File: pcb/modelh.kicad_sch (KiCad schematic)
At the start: 46 parts, among them J1 Battery Conn, J2 Conn_01x20, J3 Conn_01x05, J4 Conn_01x12, J5 Conn_01x04, J6 Conn_01x04, SW1 SW_reset, U1 nice_nano, U2 74HC595, U3 74HC595, U4 74HC595

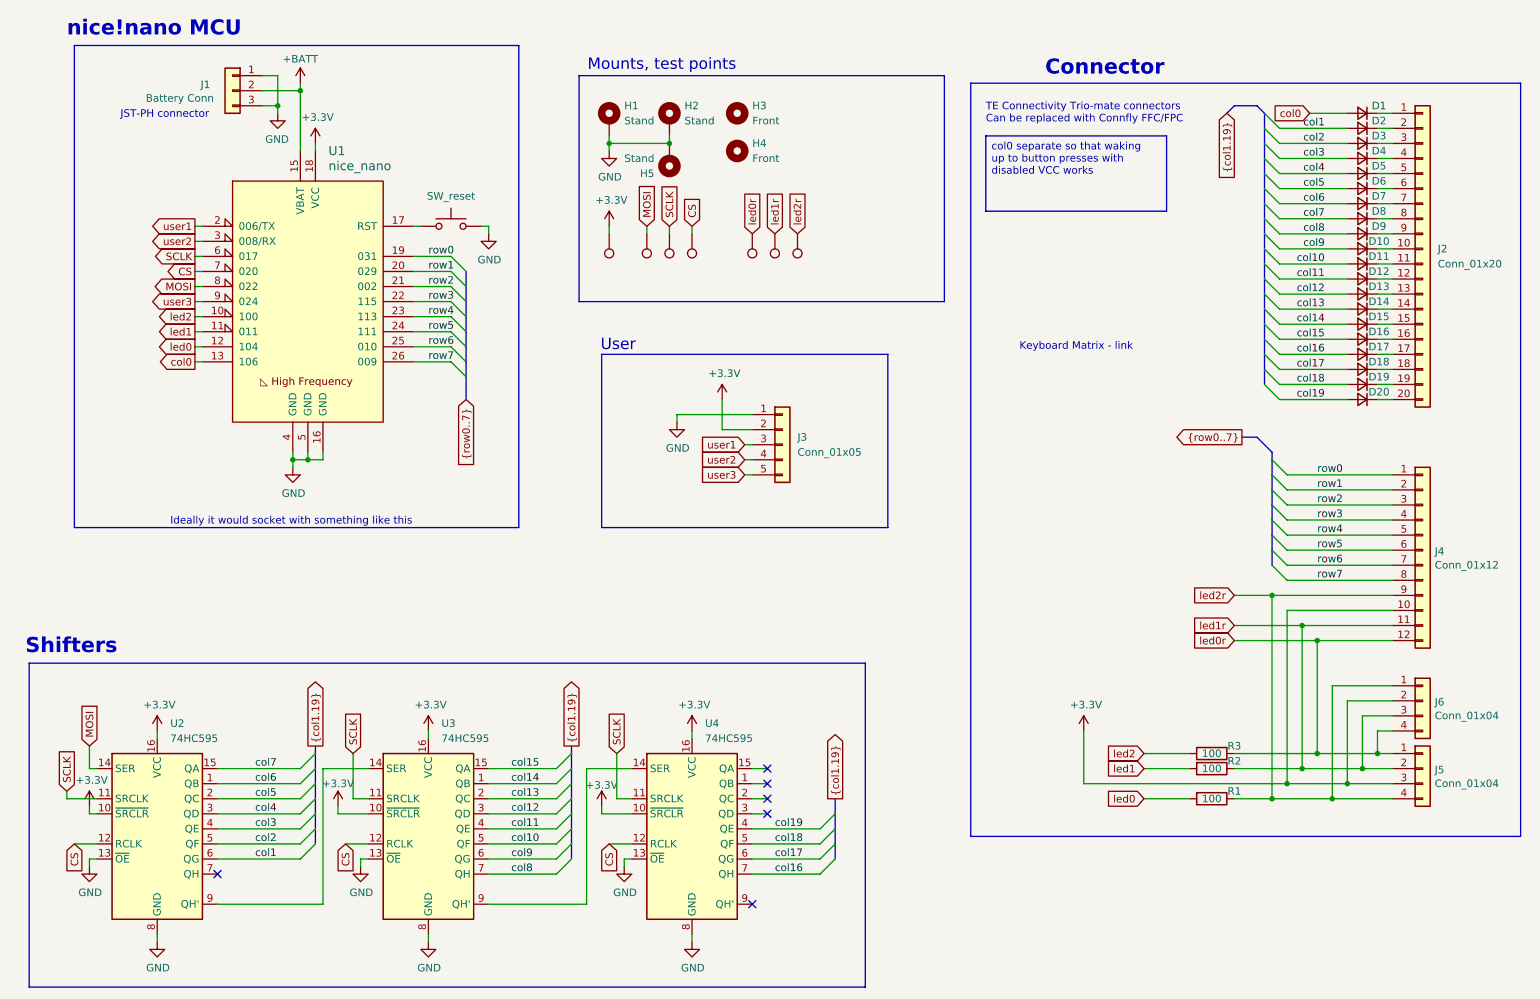
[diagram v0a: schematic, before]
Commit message: v0.7, too much to comment
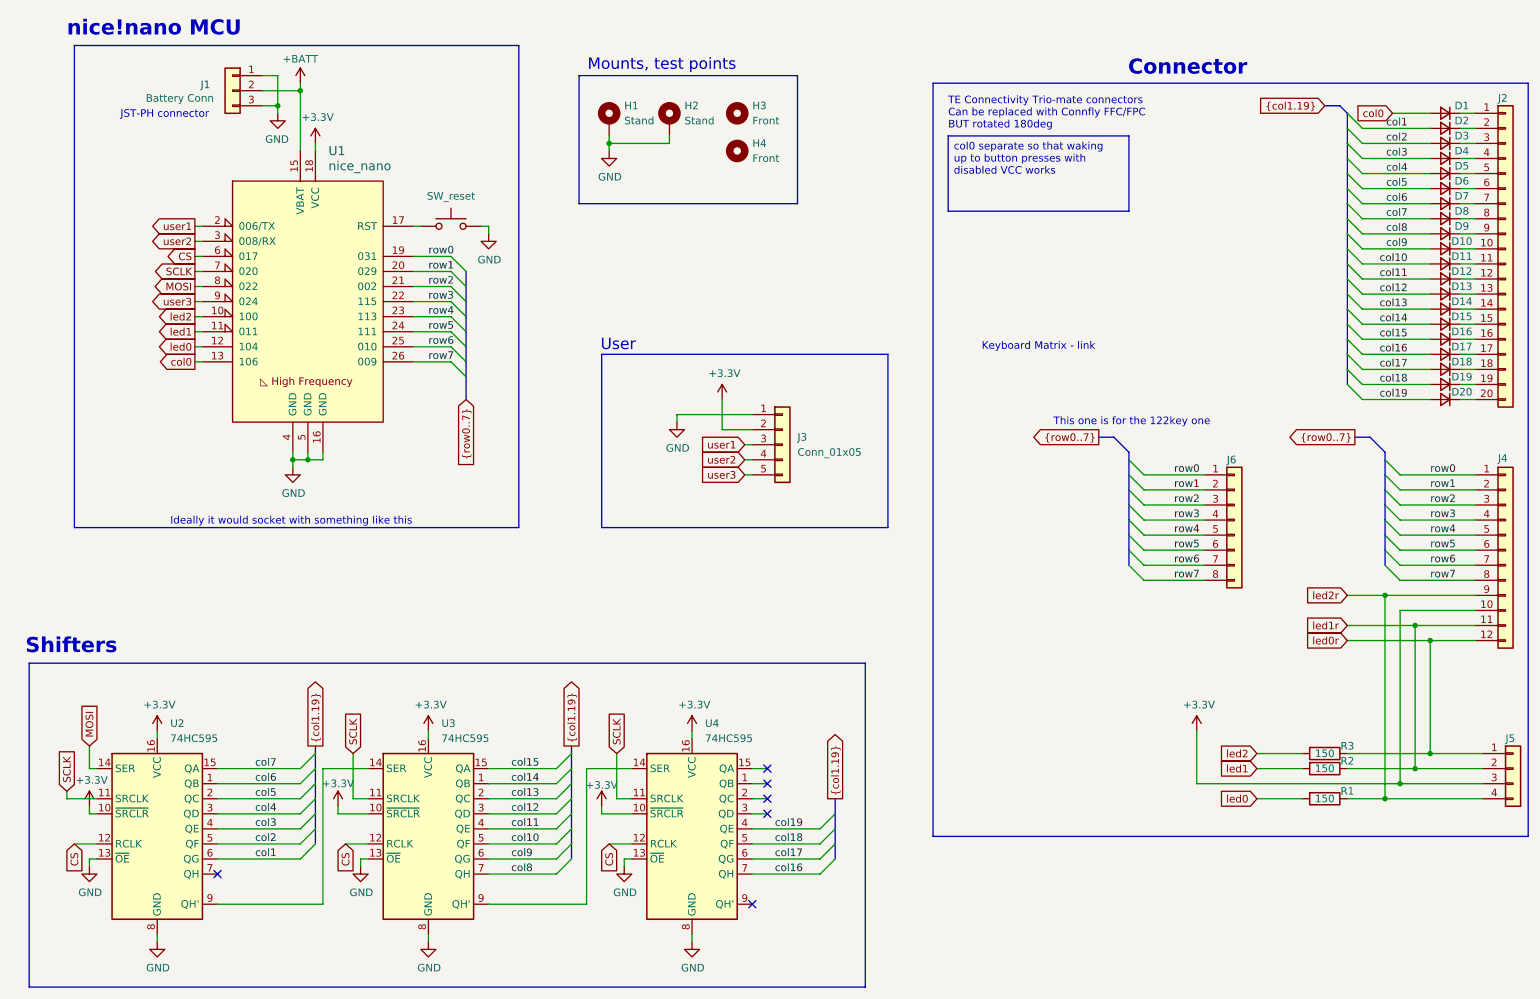
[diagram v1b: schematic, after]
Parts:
- removed H5: Stand, MountingHole:MountingHole_4mm_Pad_Via, symbol Mechanical:MountingHole_Pad
- removed J6: Conn_01x04, Library:ModelH-triomate-leds4, symbol Connector_Generic:Conn_01x04
- removed TP1: VCC, TestPoint:TestPoint_Pad_D2.5mm, symbol Connector:TestPoint
- removed TP2: MOSI, Library:TestPoint, symbol Connector:TestPoint
- removed TP3: SCLK, Library:TestPoint, symbol Connector:TestPoint
- removed TP4: CS, Library:TestPoint, symbol Connector:TestPoint
- removed TP5: LED0, Library:TestPoint, symbol Connector:TestPoint
- removed TP6: LED1, Library:TestPoint, symbol Connector:TestPoint
- removed TP7: LED2, Library:TestPoint, symbol Connector:TestPoint
- added J6: Conn_01x08, Library:ModelH-triomate-rows8, symbol Connector_Generic:Conn_01x08
- R1, R2, R3: value 100 -> 150
- U2, U3, U4: footprint Package_DIP:DIP-16_W7.62mm_Socket_LongPads -> Library:DIP-16-74HC595
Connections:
- net CS: now also U1.6 (017); no longer U1.7 (020)
- net SCLK: now also U1.7 (020); no longer U1.6 (017)
- net row0: now also J6.1 (Pin_1)
- net row1: now also J6.2 (Pin_2)
- net row2: now also J6.3 (Pin_3)
- net row3: now also J6.4 (Pin_4)
- net row4: now also J6.5 (Pin_5)
- net row5: now also J6.6 (Pin_6)
- net row6: now also J6.7 (Pin_7)
- net row7: now also J6.8 (Pin_8)
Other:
- note added: "TE Connectivity Trio-mate connectors Can be replaced with Connfly FFC/FPC BUT rotated 180deg"
- note added: "This one is for the 122key one"
- note removed: "TE Connectivity Trio-mate connectors Can be replaced with Connfly FFC/FPC"
- moved on the sheet: D1, D10, D11, D12, D13, D14, D15, D16, D17, D18, D19, D2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
